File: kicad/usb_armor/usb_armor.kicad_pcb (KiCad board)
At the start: 2 copper layers, 2 parts

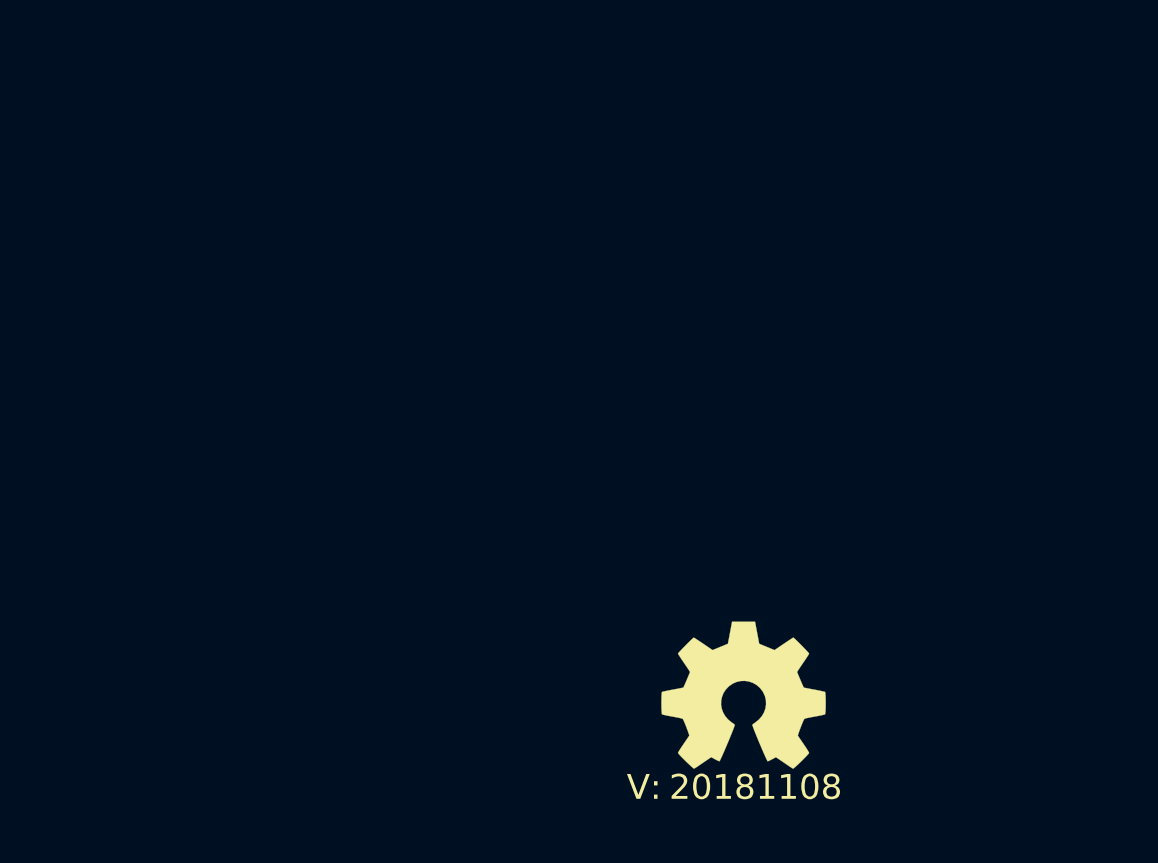
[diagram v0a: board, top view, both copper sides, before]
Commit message: initial placement completed
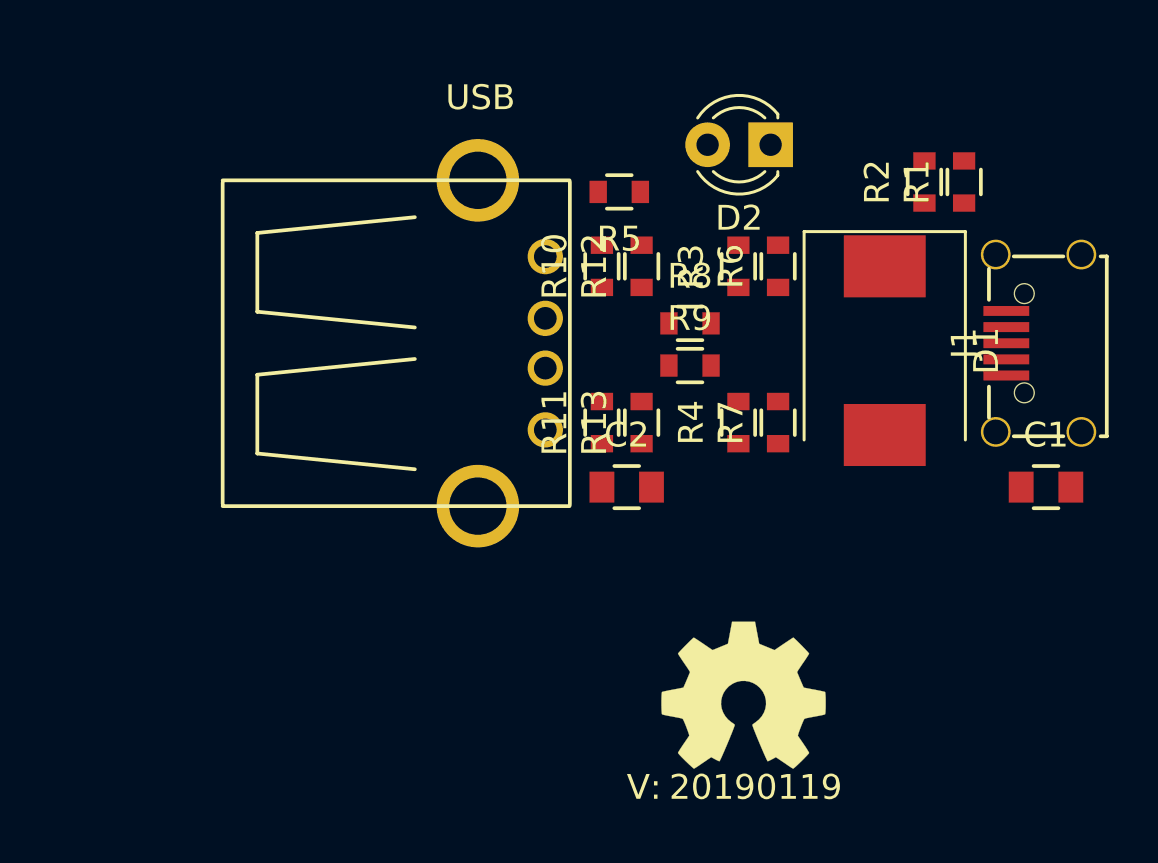
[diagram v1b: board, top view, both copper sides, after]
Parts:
- added C1: 10n, SquantorRcl:C_0805, F.Cu at (160.2, 92.6)
- added C2: 2.2u, SquantorRcl:C_0805, F.Cu at (143.3, 92.6)
- added D1: 5V_TVS, Diode_SMD:D_SMC, F.Cu at (153.7, 87.1)
- added D2: LED, LED_THT:LED_D3.0mm, F.Cu at (149.1, 78.8)
- added J1: USB-ID, SquantorUsb:USB-muB-SMD_TH, F.Cu at (159.9, 86.8)
- added J2: USB, SquantorUsb:USB-A-TH, F.Cu at (137.3, 86.8)
- added R1: R, SquantorRcl:R_0603_hand, F.Cu at (156.9, 80.3)
- added R10: TBD, SquantorRcl:R_0603_hand, F.Cu at (142.3, 83.7)
- added R11: TBD, SquantorRcl:R_0603_hand, F.Cu at (142.3, 90.0)
- added R12: TBD, SquantorRcl:R_0603_hand, F.Cu at (143.9, 83.7)
- added R13: TBD, SquantorRcl:R_0603_hand, F.Cu at (143.9, 90.0)
- added R2: R, SquantorRcl:R_0603_hand, F.Cu at (155.3, 80.3)
- added R3: TBD, SquantorRcl:R_0603_hand, F.Cu at (147.8, 83.7)
- added R4: TBD, SquantorRcl:R_0603_hand, F.Cu at (147.8, 90.0)
- added R5: 1K, SquantorRcl:R_0603_hand, F.Cu at (143.0, 80.7)
- added R6: TBD, SquantorRcl:R_0603_hand, F.Cu at (149.4, 83.7)
- added R7: TBD, SquantorRcl:R_0603_hand, F.Cu at (149.4, 90.0)
- added R8: 0, SquantorRcl:R_0603_hand, F.Cu at (145.8, 86.0)
- added R9: 0, SquantorRcl:R_0603_hand, F.Cu at (145.8, 87.7)
- N2: value 20181108 -> 20190119

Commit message: further layout
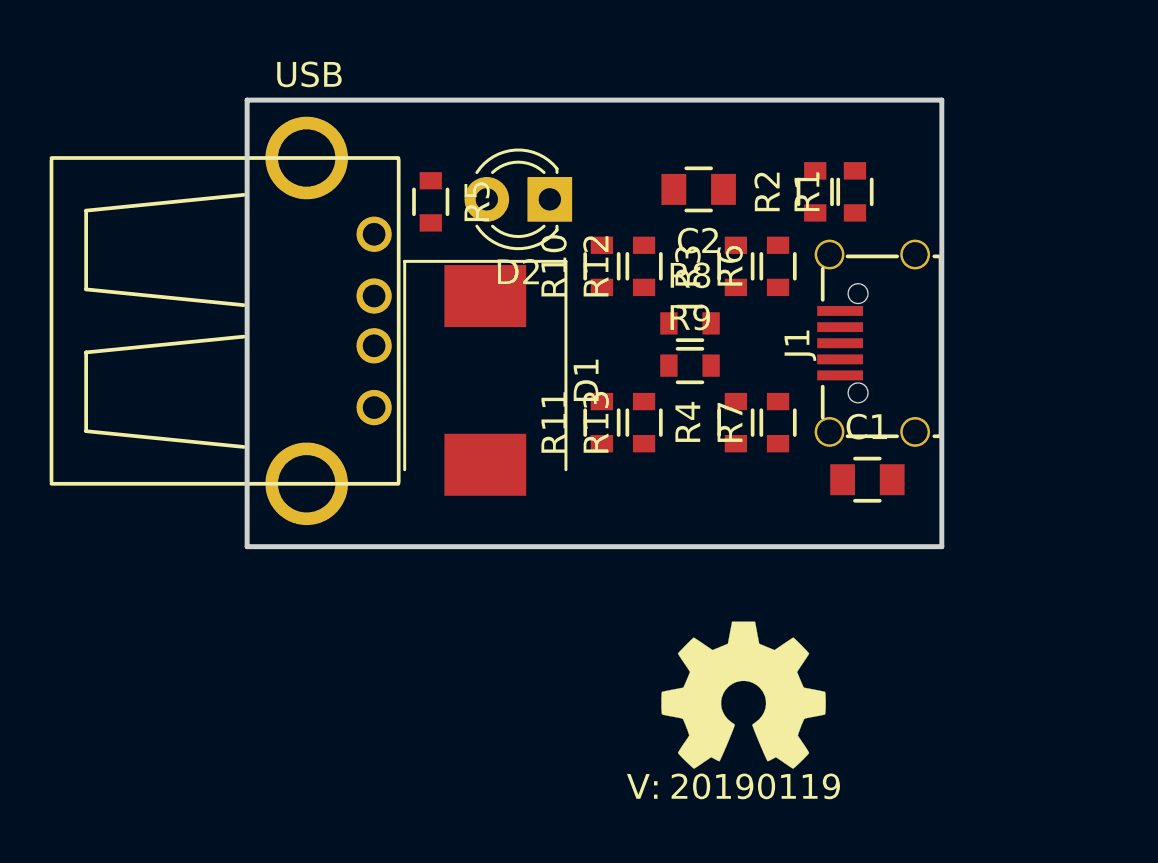
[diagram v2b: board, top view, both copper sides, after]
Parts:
- moved D1 16.1 mm to (137.6, 88.3)
- moved C2 12.3 mm to (146.2, 80.6), turned to 180 degrees
- moved D2 9.17 mm to (140.2, 81.0)
- moved R5 7.61 mm to (135.4, 81.1), turned to 270 degrees
- moved C1 7.21 mm to (153.0, 92.3)
- moved J2 6.96 mm to (130.4, 85.9)
- moved J1 6.70 mm to (153.2, 86.8)
- moved R1 4.42 mm to (152.5, 80.7)
- moved R2 4.42 mm to (150.9, 80.7)
- moved R3 0.10 mm to (147.7, 83.7)
- moved R4 0.10 mm to (147.7, 90.0)
- moved R12 0.10 mm to (144.0, 83.7)
- moved R13 0.10 mm to (144.0, 90.0)
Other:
- board outline added: 28 x 18 mm
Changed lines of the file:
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@@
   (general
     (thickness 1.6)
-    (drawings 0)
+    (drawings 4)
     (tracks 0)
     (zones 0)
@@
   )
   (module SquantorRcl:C_0805 (layer F.Cu)
-    (at 160.2 92.6)
+    (at 153 92.3)
     (descr "Capacitor SMD 0805, reflow soldering, AVX (see smccp.pdf)")
     (tags "capacitor 0805")
@@
   )
   (module SquantorRcl:C_0805 (layer F.Cu)
-    (at 143.3 92.6)
+    (at 146.2 80.6 180)
     (descr "Capacitor SMD 0805, reflow soldering, AVX (see smccp.pdf)")
     (tags "capacitor 0805")
     (attr smd)
-    (fp_text reference C2 (at 0 -2.1) (layer F.SilkS)
-      (effects (font (size 1 1) (thickness 0.15)))
-    )
-    (fp_text value 2.2u (at 0 2.1) (layer F.Fab)
+    (fp_text reference C2 (at 0 -2.1 180) (layer F.SilkS)
+      (effects (font (size 1 1) (thickness 0.15)))
+    )
+    (fp_text value 2.2u (at 0 2.1 180) (layer F.Fab)
       (effects (font (size 1 1) (thickness 0.15)))
     )
@@
     (fp_line (start 1 0.625) (end -1 0.625) (layer F.Fab) (width 0.15))
     (fp_line (start -1 0.625) (end -1 -0.625) (layer F.Fab) (width 0.15))
-    (pad 2 smd rect (at 1 0) (size 1 1.25) (layers F.Cu F.Paste F.Mask)
-      (net 3 VCC))
-    (pad 1 smd rect (at -1 0) (size 1 1.25) (layers F.Cu F.Paste F.Mask)
+    (pad 2 smd rect (at 1 0 180) (size 1 1.25) (layers F.Cu F.Paste F.Mask)
+      (net 3 VCC))
+    (pad 1 smd rect (at -1 0 180) (size 1 1.25) (layers F.Cu F.Paste F.Mask)
       (net 1 GND))
     (model Capacitors_SMD.3dshapes/C_0805.wrl
@@
   )
   (module Diode_SMD:D_SMC (layer F.Cu)
-    (at 153.7 87.1 270)
+    (at 137.6 88.3 270)
     (descr "Diode SMC (DO-214AB)")
     (tags "Diode SMC (DO-214AB)")
@@
   )
   (module LED_THT:LED_D3.0mm (layer F.Cu)
-    (at 149.1 78.8 180)
+    (at 140.2 81 180)
     (descr "LED, diameter 3.0mm, 2 pins")
     (tags "LED diameter 3.0mm 2 pins")
@@
   )
   (module SquantorUsb:USB-muB-SMD_TH (layer F.Cu)
-    (at 159.9 86.8 90)
+    (at 153.2 86.8 90)
     (fp_text reference J1 (at 0 -3 90) (layer F.SilkS)
       (effects (font (size 1 1) (thickness 0.15)))
@@
   )
   (module SquantorUsb:USB-A-TH (layer F.Cu)
-    (at 137.3 86.8)
+    (at 130.4 85.9)
     (descr "USB SERIES A HOLE MOUNTED")
     (tags "USB SERIES A HOLE MOUNTED")
@@
   )
   (module SquantorRcl:R_0603_hand (layer F.Cu)
-    (at 156.9 80.3 90)
+    (at 152.5 80.7 90)
     (descr "Resistor SMD 0603, reflow soldering, Vishay (see dcrcw.pdf)")
     (tags "resistor 0603")
@@
   )
   (module SquantorRcl:R_0603_hand (layer F.Cu)
-    (at 155.3 80.3 90)
+    (at 150.9 80.7 90)
     (descr "Resistor SMD 0603, reflow soldering, Vishay (see dcrcw.pdf)")
     (tags "resistor 0603")
@@
   )
   (module SquantorRcl:R_0603_hand (layer F.Cu)
-    (at 147.8 83.7 90)
+    (at 147.7 83.7 90)
     (descr "Resistor SMD 0603, reflow soldering, Vishay (see dcrcw.pdf)")
     (tags "resistor 0603")
@@
   )
   (module SquantorRcl:R_0603_hand (layer F.Cu)
-    (at 147.8 90 90)
+    (at 147.7 90 90)
     (descr "Resistor SMD 0603, reflow soldering, Vishay (see dcrcw.pdf)")
     (tags "resistor 0603")
@@
   )
   (module SquantorRcl:R_0603_hand (layer F.Cu)
-    (at 143 80.7 180)
-    (descr "Resistor SMD 0603, reflow soldering, Vishay (see dcrcw.pdf)")
-    (tags "resistor 0603")
-    (attr smd)
-    (fp_text reference R5 (at 0 -1.9 180) (layer F.SilkS)
-      (effects (font (size 1 1) (thickness 0.15)))
-    )
-    (fp_text value 1K (at 0 1.9 180) (layer F.Fab)
-      (effects (font (size 1 1) (thickness 0.15)))
-    )
-    (fp_line (start -0.5 -0.675) (end 0.5 -0.675) (layer F.SilkS) (width 0.15))
-    (fp_line (start 0.5 0.675) (end -0.5 0.675) (layer F.SilkS) (width 0.15))
-    (fp_line (start 1.5 -0.8) (end 1.5 0.8) (layer F.CrtYd) (width 0.05))
-    (fp_line (start -1.5 -0.8) (end -1.5 0.8) (layer F.CrtYd) (width 0.05))
-    (fp_line (start -1.5 0.8) (end 1.5 0.8) (layer F.CrtYd) (width 0.05))
-    (fp_line (start -1.5 -0.8) (end 1.5 -0.8) (layer F.CrtYd) (width 0.05))
-    (fp_line (start -0.8 -0.4) (end 0.8 -0.4) (layer F.Fab) (width 0.1))
-    (fp_line (start 0.8 -0.4) (end 0.8 0.4) (layer F.Fab) (width 0.1))
-    (fp_line (start 0.8 0.4) (end -0.8 0.4) (layer F.Fab) (width 0.1))
-    (fp_line (start -0.8 0.4) (end -0.8 -0.4) (layer F.Fab) (width 0.1))
-    (pad 2 smd rect (at 0.85 0 180) (size 0.7 0.9) (layers F.Cu F.Paste F.Mask)
-      (net 3 VCC))
-    (pad 1 smd rect (at -0.85 0 180) (size 0.7 0.9) (layers F.Cu F.Paste F.Mask)
+    (at 135.4 81.1 270)
+    (descr "Resistor SMD 0603, reflow soldering, Vishay (see dcrcw.pdf)")
+    (tags "resistor 0603")
+    (attr smd)
+    (fp_text reference R5 (at 0 -1.9 270) (layer F.SilkS)
+      (effects (font (size 1 1) (thickness 0.15)))
+    )
+    (fp_text value 1K (at 0 1.9 270) (layer F.Fab)
+      (effects (font (size 1 1) (thickness 0.15)))
+    )
+    (fp_line (start -0.5 -0.675) (end 0.5 -0.675) (layer F.SilkS) (width 0.15))
+    (fp_line (start 0.5 0.675) (end -0.5 0.675) (layer F.SilkS) (width 0.15))
+    (fp_line (start 1.5 -0.8) (end 1.5 0.8) (layer F.CrtYd) (width 0.05))
+    (fp_line (start -1.5 -0.8) (end -1.5 0.8) (layer F.CrtYd) (width 0.05))
+    (fp_line (start -1.5 0.8) (end 1.5 0.8) (layer F.CrtYd) (width 0.05))
+    (fp_line (start -1.5 -0.8) (end 1.5 -0.8) (layer F.CrtYd) (width 0.05))
+    (fp_line (start -0.8 -0.4) (end 0.8 -0.4) (layer F.Fab) (width 0.1))
+    (fp_line (start 0.8 -0.4) (end 0.8 0.4) (layer F.Fab) (width 0.1))
+    (fp_line (start 0.8 0.4) (end -0.8 0.4) (layer F.Fab) (width 0.1))
+    (fp_line (start -0.8 0.4) (end -0.8 -0.4) (layer F.Fab) (width 0.1))
+    (pad 2 smd rect (at 0.85 0 270) (size 0.7 0.9) (layers F.Cu F.Paste F.Mask)
+      (net 3 VCC))
+    (pad 1 smd rect (at -0.85 0 270) (size 0.7 0.9) (layers F.Cu F.Paste F.Mask)
       (net 4 "Net-(D2-Pad2)"))
     (model Resistors_SMD.3dshapes/R_0603.wrl
@@
   )
   (module SquantorRcl:R_0603_hand (layer F.Cu)
-    (at 143.9 83.7 90)
+    (at 144 83.7 90)
     (descr "Resistor SMD 0603, reflow soldering, Vishay (see dcrcw.pdf)")
     (tags "resistor 0603")
@@
   )
   (module SquantorRcl:R_0603_hand (layer F.Cu)
-    (at 143.9 90 90)
+    (at 144 90 90)
     (descr "Resistor SMD 0603, reflow soldering, Vishay (see dcrcw.pdf)")
     (tags "resistor 0603")
@@
     )
   )
+  (gr_line (start 156 77) (end 128 77) (layer Edge.Cuts) (width 0.2))
+  (gr_line (start 156 95) (end 156 77) (layer Edge.Cuts) (width 0.2))
+  (gr_line (start 128 95) (end 156 95) (layer Edge.Cuts) (width 0.2))
+  (gr_line (start 128 77) (end 128 95) (layer Edge.Cuts) (width 0.2))
 )
